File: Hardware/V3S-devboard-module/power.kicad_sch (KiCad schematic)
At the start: 56 parts, among them U101 EA3036C, U102 XC6206PxxxMR

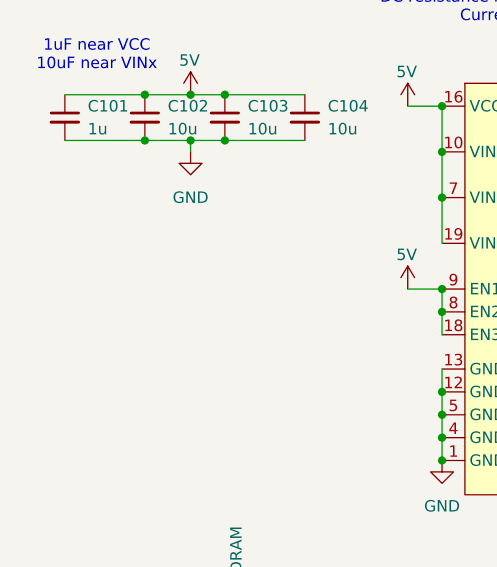
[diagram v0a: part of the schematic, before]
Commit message: layout
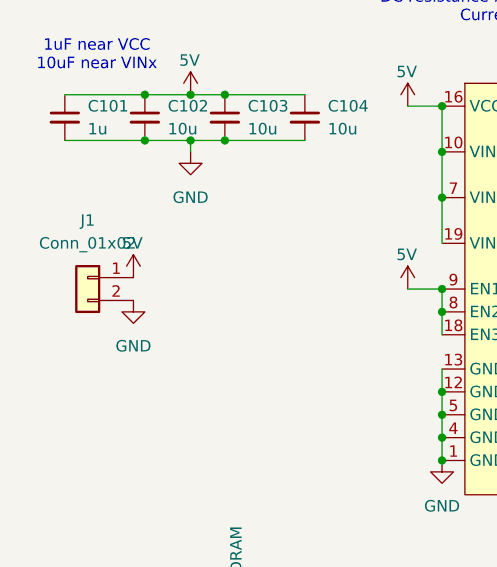
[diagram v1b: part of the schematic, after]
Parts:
- added J1: Conn_01x02, Connector_PinHeader_2.54mm:PinHeader_1x02_P2.54mm_Vertical, symbol Connector_Generic:Conn_01x02
- U101: LCSC (none) -> C570857; LCSC Part C570857 -> (none)
- U102: LCSC (none) -> C5148691
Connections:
- net 5V: now also J1.1 (Pin_1)
- net GND: now also J1.2 (Pin_2)
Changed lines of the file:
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@@
 	)
 	(symbol
+		(lib_id "Connector_Generic:Conn_01x02")
+		(at 27.94 57.15 0)
+		(mirror y)
+		(unit 1)
+		(exclude_from_sim no)
+		(in_bom yes)
+		(on_board yes)
+		(dnp no)
+		(fields_autoplaced yes)
+		(property "Reference" "J1"
+			(at 27.94 50.8 0)
+			(effects
+				(font
+					(size 1.27 1.27)
+				)
+			)
+		)
+		(property "Value" "Conn_01x02"
+			(at 27.94 53.34 0)
+			(effects
+				(font
+					(size 1.27 1.27)
+				)
+			)
+		)
+		(property "Footprint" "Connector_PinHeader_2.54mm:PinHeader_1x02_P2.54mm_Vertical"
+			(at 27.94 57.15 0)
+			(effects
+				(font
+					(size 1.27 1.27)
+				)
+				(hide yes)
+			)
+		)
+		(property "Datasheet" "~"
+			(at 27.94 57.15 0)
+			(effects
+				(font
+					(size 1.27 1.27)
+				)
+				(hide yes)
+			)
+		)
+		(property "Description" "Generic connector, single row, 01x02, script generated (kicad-library-utils/schlib/autogen/connector/)"
+			(at 27.94 57.15 0)
+			(effects
+				(font
+					(size 1.27 1.27)
+				)
+				(hide yes)
+			)
+		)
+		(pin "1"
+		)
+		(pin "2"
+		)
+		(instances
+			(project "V3S-devboard-module"
+				(path "/5d41c08e-2331-42df-a2d5-1aeb6ed4388c/5949d9b7-76b3-40a2-8931-5cd58c7934ef"
+					(reference "J1")
+					(unit 1)
+				)
+			)
+		)
+	)
+	(symbol
 		(lib_id "power:GND")
 		(at 140.97 63.5 0)
@@
 			)
 		)
+		(property "LCSC" "C5148691"
+			(at 176.53 39.37 0)
+			(effects
+				(font
+					(size 1.27 1.27)
+				)
+				(hide yes)
+			)
+		)
 		(pin "2"
 		)
@@
 	)
 	(symbol
+		(lib_id "power:VCC")
+		(at 33.02 57.15 0)
+		(unit 1)
+		(exclude_from_sim no)
+		(in_bom yes)
+		(on_board yes)
+		(dnp no)
+		(property "Reference" "#PWR0108"
+			(at 33.02 60.96 0)
+			(effects
+				(font
+					(size 1.27 1.27)
+				)
+				(hide yes)
+			)
+		)
+		(property "Value" "5V"
+			(at 31.75 53.34 0)
+			(effects
+				(font
+					(size 1.27 1.27)
+				)
+				(justify left)
+			)
+		)
+		(property "Footprint" ""
+			(at 33.02 57.15 0)
+			(effects
+				(font
+					(size 1.27 1.27)
+				)
+				(hide yes)
+			)
+		)
+		(property "Datasheet" ""
+			(at 33.02 57.15 0)
+			(effects
+				(font
+					(size 1.27 1.27)
+				)
+				(hide yes)
+			)
+		)
+		(property "Description" "Power symbol creates a global label with name \"VCC\""
+			(at 33.02 57.15 0)
+			(effects
+				(font
+					(size 1.27 1.27)
+				)
+				(hide yes)
+			)
+		)
+		(pin "1"
+		)
+		(instances
+			(project "V3S-devboard-module"
+				(path "/5d41c08e-2331-42df-a2d5-1aeb6ed4388c/5949d9b7-76b3-40a2-8931-5cd58c7934ef"
+					(reference "#PWR0108")
+					(unit 1)
+				)
+			)
+		)
+	)
+	(symbol
 		(lib_id "Device:C_Small")
 		(at 147.32 144.78 180)
@@
 	)
 	(symbol
+		(lib_id "power:GND")
+		(at 33.02 59.69 0)
+		(unit 1)
+		(exclude_from_sim no)
+		(in_bom yes)
+		(on_board yes)
+		(dnp no)
+		(fields_autoplaced yes)
+		(property "Reference" "#PWR0122"
+			(at 33.02 66.04 0)
+			(effects
+				(font
+					(size 1.27 1.27)
+				)
+				(hide yes)
+			)
+		)
+		(property "Value" "GND"
+			(at 33.02 64.77 0)
+			(effects
+				(font
+					(size 1.27 1.27)
+				)
+			)
+		)
+		(property "Footprint" ""
+			(at 33.02 59.69 0)
+			(effects
+				(font
+					(size 1.27 1.27)
+				)
+				(hide yes)
+			)
+		)
+		(property "Datasheet" ""
+			(at 33.02 59.69 0)
+			(effects
+				(font
+					(size 1.27 1.27)
+				)
+				(hide yes)
+			)
+		)
+		(property "Description" "Power symbol creates a global label with name \"GND\" , ground"
+			(at 33.02 59.69 0)
+			(effects
+				(font
+					(size 1.27 1.27)
+				)
+				(hide yes)
+			)
+		)
+		(pin "1"
+		)
+		(instances
+			(project "V3S-devboard-module"
+				(path "/5d41c08e-2331-42df-a2d5-1aeb6ed4388c/5949d9b7-76b3-40a2-8931-5cd58c7934ef"
+					(reference "#PWR0122")
+					(unit 1)
+				)
+			)
+		)
+	)
+	(symbol
 		(lib_id "Device:C_Small")
 		(at 54.61 111.76 180)
@@
 			)
 		)
-		(property "LCSC Part" "C570857"
+		(property "LCSC" "C570857"
 			(at 78.74 81.28 0)
 			(effects
